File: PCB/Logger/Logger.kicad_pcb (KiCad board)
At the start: 2 copper layers, 70 x 70 mm, 68 parts, among them J1 JST-PH-SM4-TB, J2 USB-C-Socket-V, J3 Conn_01x05, J4 Shelly, J5 USB-PROG, J6 TF_PUSH, Q1 CJ2301, Q2 C179347, U1 ESP32-S3-MINI-1, U3 TP4054, U4 ME6211C33M5G-N

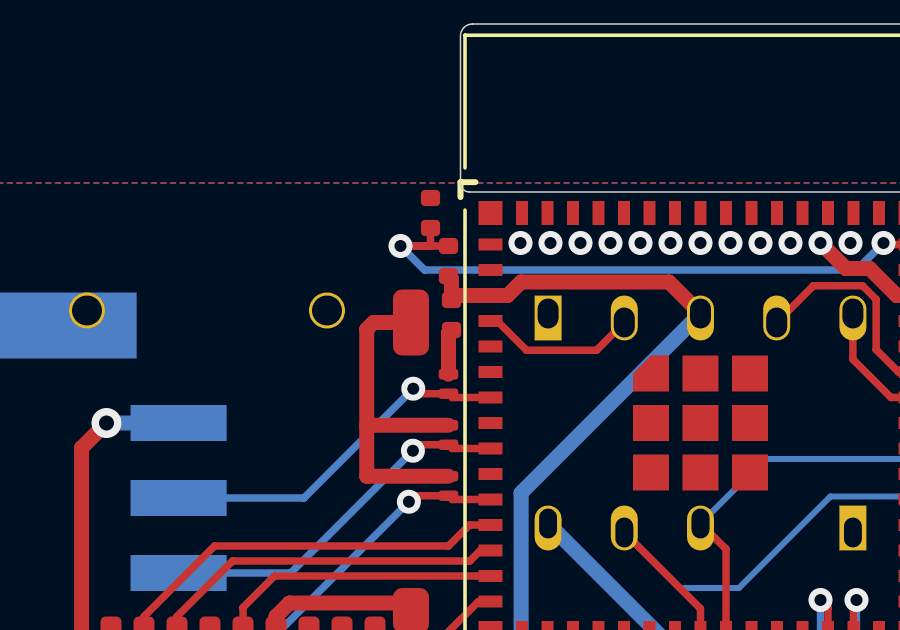
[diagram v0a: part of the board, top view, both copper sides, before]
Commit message: Tidy
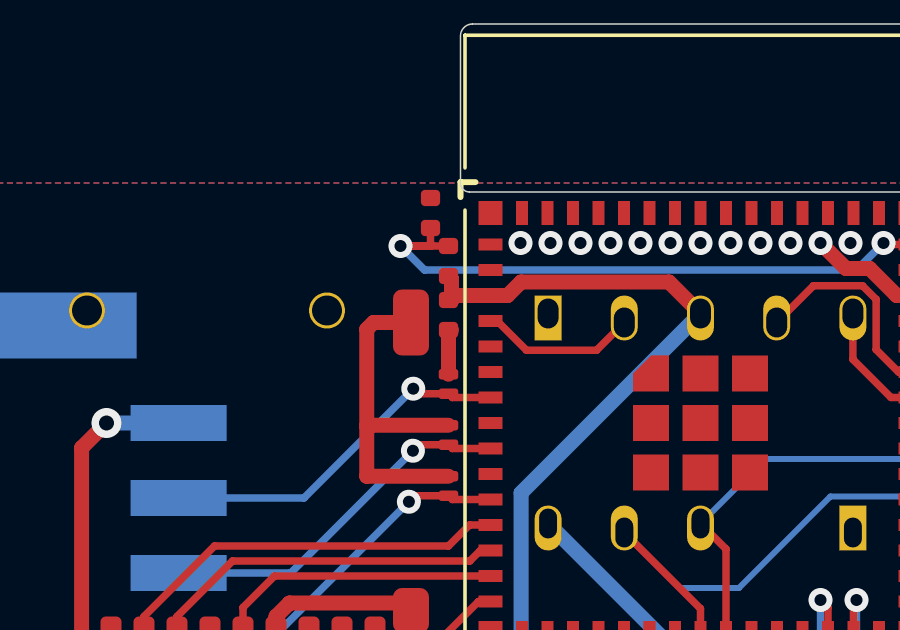
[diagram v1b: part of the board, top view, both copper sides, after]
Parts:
- moved C19 0.10 mm to (95.6, 94.4)
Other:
- board text added: "C"
- board text added: "S"
